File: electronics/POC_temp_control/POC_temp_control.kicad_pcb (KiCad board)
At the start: 2 copper layers, 109.2 x 78.7 mm, 177 parts, among them J1 Conn_01x02, J2 Conn_01x07, J3 Conn_01x05, J4 Conn_01x06, J5 Conn_01x02, J6 Conn_01x02, Q1 PXT8050, Q2 PXT8050, Q3 PXT8550, Q4 Q_PMOS_DUAL, Q5 BC858B, Q6 BC847A, Q7 Q_PMOS_DUAL, Q8 BC858B, Q9 BC847A, T1 10P_1P_2S, U1 SY8120, U2 MCP1702T-3302, U4 LM358, U5 OP07, U6 OP07, U7 OP07, U8 74XX4051, U9 74XX4051

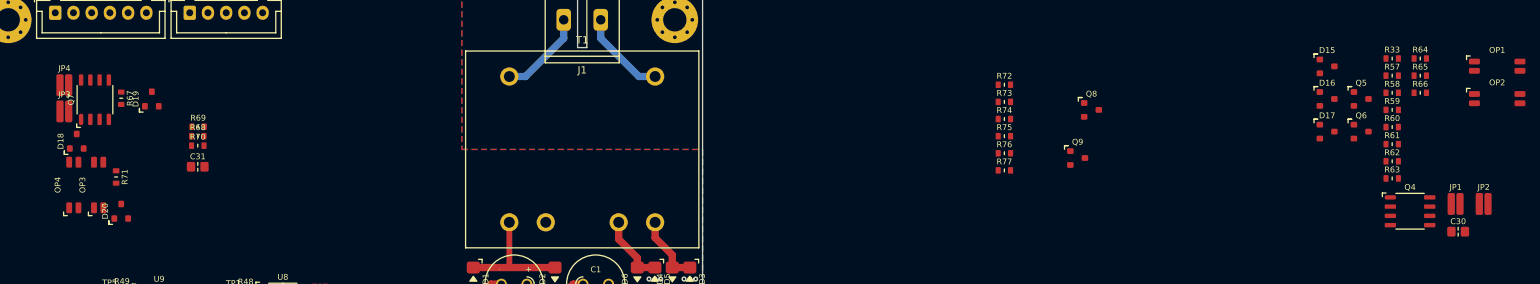
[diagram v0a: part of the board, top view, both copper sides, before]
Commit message: straggling changes
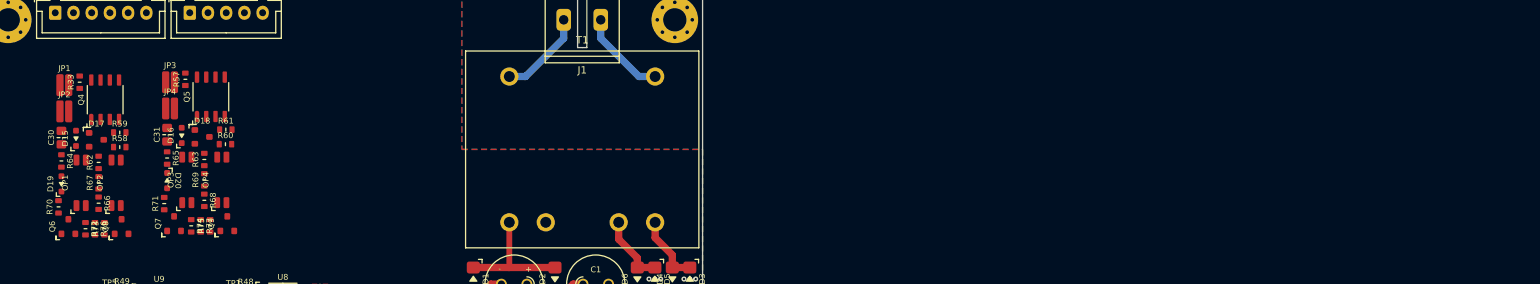
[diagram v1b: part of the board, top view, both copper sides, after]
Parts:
- D15: value BZX84C18 -> BZT52C18; footprint SquantorIC:SOT23-3 -> SquantorDiodes:SOD-323-nexperia-hand
- D16: value BAV70 -> BZT52C18; footprint SquantorIC:SOT23-3 -> SquantorDiodes:SOD-323-nexperia-hand
- D17: value BAS16 -> BAV70
- D18: value BZX84C18 -> BAV70
- D19: value BAV70 -> BAS316; footprint SquantorIC:SOT23-3 -> SquantorDiodes:SOD-323-nexperia-hand
- D20: value BAS16 -> BAS316; footprint SquantorIC:SOT23-3 -> SquantorDiodes:SOD-323-nexperia-hand
- Q5: value BC858B -> Q_PMOS_DUAL; footprint SquantorIC:SOT23-3 -> SquantorIC:SOIC-8
- Q6: value BC847A -> BC858B
- Q7: value Q_PMOS_DUAL -> BC858B; footprint SquantorIC:SOIC-8 -> SquantorIC:SOT23-3
- Q8: value BC858B -> BC847A
- R57: value 5K6 -> 10M
- R58: value 1M -> 5K6
- R59: value 1K5 -> 1M
- R60: value 2K2 -> 5K6
- R61: value 330 -> 1M
- R62: value 330 -> 1K5
- R63: value 6K8 -> 1K5
- R64, R65: value 10K -> 2K2
- R66: value 10K -> 330
- R67: value 10M -> 330
- R68: value 5K6 -> 330
- R69: value 1M -> 330
- R70: value 1K5 -> 6K8
- R71: value 2K2 -> 6K8
- R72, R73: value 330 -> 10K
- R74: value 6K8 -> 10K
- moved JP2 195.1 mm to (45.8, 40.5)
- moved OP1 194.9 mm to (48.1, 50.3), turned to 90 degrees
- moved C30 192.0 mm to (45.4, 44.1), turned to 90 degrees
- moved JP1 191.5 mm to (45.8, 36.9)
- moved OP2 189.8 mm to (52.9, 50.3), turned to 90 degrees
- moved R64 186.9 mm to (45.4, 47.3), turned to -90 degrees
- moved R66 181.9 mm to (50.5, 53.1), turned to -90 degrees
- moved R33 180.1 mm to (47.9, 36.5), turned to 90 degrees
- moved Q4 179.7 mm to (51.4, 38.9), turned to 90 degrees
- moved Q6 177.8 mm to (46.4, 56.3), turned to 90 degrees
- moved R62 177.5 mm to (50.5, 47.5), turned to 90 degrees
- moved R58 174.7 mm to (53.4, 45.4)
- moved R59 174.6 mm to (53.4, 43.4)
- moved R65 172.3 mm to (59.9, 46.9), turned to -90 degrees
- moved D15 171.9 mm to (47.4, 44.2), turned to 90 degrees
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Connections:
- net /Power control/AC_P1 renamed /AC_P1
- C30 pad 2: /Power control/SW_S1 -> /SW_S1
- C31 pad 1: Net-(D18-K) -> Net-(D16-K)
- C31 pad 2: /Power control/SW_S2 -> /SW_S2
- D15 pad 1: /Power control/SW_S1 -> Net-(D15-K)
- D15 pad 2: (no net) -> /SW_S1
- D16 pad 1: /Power control/SW_S1 -> Net-(D16-K)
- D16 pad 2: Net-(D16-K2) -> /SW_S2
- D17 pad 1: /Power control/GND -> /SW_S1
- D17 pad 2: (no net) -> Net-(D17-K2)
- D17 pad 3: Net-(D17-K) -> /SW_G1
- D18 pad 1: /Power control/SW_S2 -> /SW_S2
- D18 pad 2: (no net) -> Net-(D18-K2)
- D18 pad 3: Net-(D18-K) -> /SW_G2
- D19 pad 1: /Power control/SW_S2 -> Net-(D19-K)
- D19 pad 2: Net-(D19-K2) -> /GND
- D20 pad 1: /Power control/GND -> Net-(D20-K)
- D20 pad 2: (no net) -> /GND
- JP1 pad 1: /Power control/AC2 -> /AC2
- JP2 pad 1: /Power control/AC1 -> /AC1
- JP3 pad 1: /Power control/AC2 -> /AC2
- JP3 pad 2: /Power control/AC_P2 -> /AC_P2
- JP4 pad 1: /Power control/AC1 -> /AC1
- JP4 pad 2: /Power control/AC_P2 -> /AC_P2
- OP1 pad 1: Net-(Q5-C) -> Net-(Q6-C)
- OP2 pad 2: Net-(Q6-C) -> Net-(Q8-C)
- OP2 pad 3: /Power control/SW_S1 -> /SW_S1
- OP2 pad 4: Net-(D16-K2) -> Net-(D17-K2)
- OP3 pad 1: Net-(Q8-C) -> Net-(Q7-C)
- OP3 pad 4: Net-(D18-K) -> Net-(D16-K)
- OP4 pad 3: /Power control/SW_S2 -> /SW_S2
- OP4 pad 4: Net-(D19-K2) -> Net-(D18-K2)
- Q4 pad 2: /Power control/SW_G1 -> /SW_G1
- Q4 pad 3: /Power control/COM1 -> /COM1
- Q4 pad 4: /Power control/SW_G1 -> /SW_G1
- Q4 pad 5: /Power control/SW_S1 -> /SW_S1
- Q4 pad 6: /Power control/SW_S1 -> /SW_S1
- Q4 pad 7: /Power control/SW_S1 -> /SW_S1
- Q4 pad 8: /Power control/SW_S1 -> /SW_S1
- Q5 pad 1: Net-(Q5-B) -> /AC_P2
- Q5 pad 2: /Power control/VD3.3V+ -> /SW_G2
- Q5 pad 3: Net-(Q5-C) -> /COM1
- Q6 pad 2: /Power control/GND -> /VD3.3V+
- Q7 pad 1: /Power control/AC_P2 -> Net-(Q7-B)
- Q7 pad 2: /Power control/SW_G2 -> /VD3.3V+
- Q7 pad 3: /Power control/COM1 -> Net-(Q7-C)
- Q8 pad 2: /Power control/VD3.3V+ -> /GND
- Q9 pad 2: /Power control/GND -> /GND
- R33 pad 2: /Power control/COM1 -> /COM1
- R57 pad 1: /Power control/SW_G1 -> /AC_P2
- R57 pad 2: Net-(D16-K2) -> /COM1
- R58 pad 1: /Power control/SW_G1 -> /SW_G1
- R58 pad 2: /Power control/SW_S1 -> Net-(D17-K2)
- R59 pad 1: Net-(OP1-Pad3) -> /SW_G1
- R59 pad 2: Net-(D16-K2) -> /SW_S1
- R60 pad 1: Net-(D15-K) -> /SW_G2
- R60 pad 2: Net-(D17-K) -> Net-(D18-K2)
- R61 pad 1: /Power control/GND -> /SW_G2
- R61 pad 2: Net-(OP1-Pad2) -> /SW_S2
- R62 pad 1: Net-(OP2-Pad1) -> Net-(OP1-Pad3)
- R62 pad 2: /Power control/VD3.3V+ -> Net-(D17-K2)
- R63 pad 1: Net-(Q5-B) -> Net-(OP3-Pad3)
- R63 pad 2: /Power control/VD3.3V+ -> Net-(D18-K2)
- R64 pad 1: Net-(Q5-B) -> Net-(D15-K)
- R64 pad 2: /Power control/SW_LOAD_1 -> Net-(D19-K)
- R65 pad 1: Net-(Q6-B) -> Net-(D16-K)
- R65 pad 2: /Power control/SW_LOAD_1 -> Net-(D20-K)
- R66 pad 1: /Power control/SW_LOAD_1 -> /GND
- R66 pad 2: /Power control/VD3.3V+ -> Net-(OP1-Pad2)
- R67 pad 1: /Power control/AC_P2 -> Net-(OP2-Pad1)
- R67 pad 2: /Power control/COM1 -> /VD3.3V+
- R68 pad 1: /Power control/SW_G2 -> /GND
- R68 pad 2: Net-(D19-K2) -> Net-(OP3-Pad2)
- R69 pad 1: /Power control/SW_G2 -> Net-(OP4-Pad1)
- R69 pad 2: /Power control/SW_S2 -> /VD3.3V+
- R70 pad 1: Net-(OP3-Pad3) -> Net-(Q6-B)
- R70 pad 2: Net-(D19-K2) -> /VD3.3V+
- R71 pad 1: Net-(D18-K) -> Net-(Q7-B)
- R71 pad 2: Net-(D20-K) -> /VD3.3V+
- R72 pad 1: /Power control/GND -> Net-(Q6-B)
- R72 pad 2: Net-(OP3-Pad2) -> /SW_LOAD_1
- R73 pad 1: Net-(OP4-Pad1) -> Net-(Q8-B)
- R73 pad 2: /Power control/VD3.3V+ -> /SW_LOAD_1
- R74 pad 1: Net-(Q8-B) -> Net-(Q7-B)
- R74 pad 2: /Power control/VD3.3V+ -> /SW_LOAD_2
- R75 pad 1: Net-(Q8-B) -> Net-(Q9-B)
- R75 pad 2: /Power control/SW_LOAD_2 -> /SW_LOAD_2
- R76 pad 1: Net-(Q9-B) -> /SW_LOAD_1
- R76 pad 2: /Power control/SW_LOAD_2 -> /VD3.3V+
- R77 pad 1: /Power control/SW_LOAD_2 -> /SW_LOAD_2
- R77 pad 2: /Power control/VD3.3V+ -> /VD3.3V+
